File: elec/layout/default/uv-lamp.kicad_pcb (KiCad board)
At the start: 2 copper layers, 21 x 21 mm, 3 parts, among them U1 ?, U2 ?, U3 ?

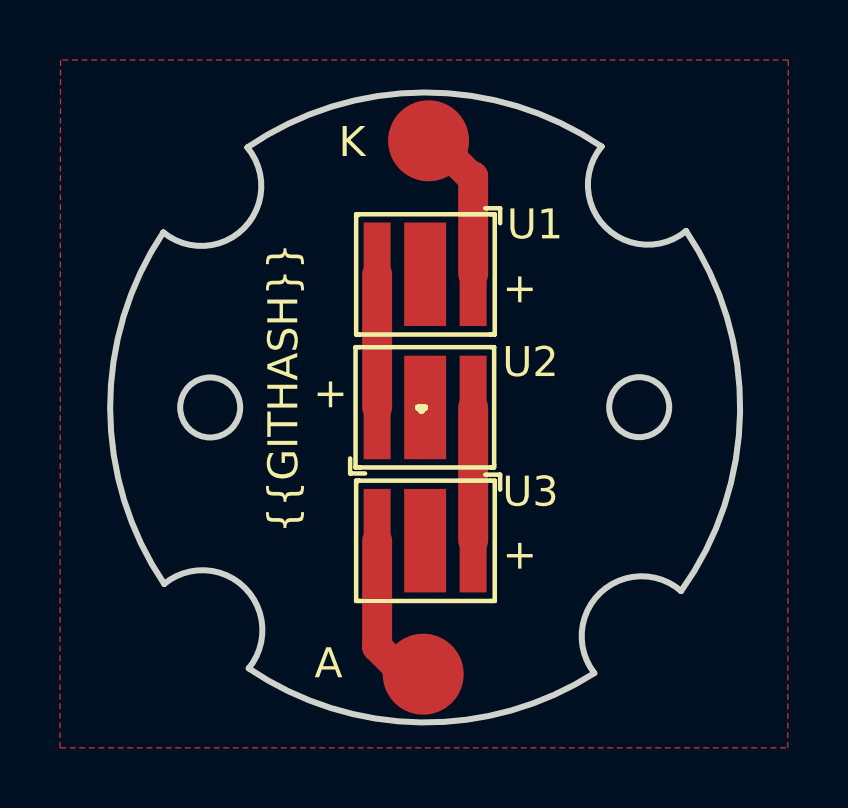
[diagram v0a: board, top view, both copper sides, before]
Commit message: ccdriver
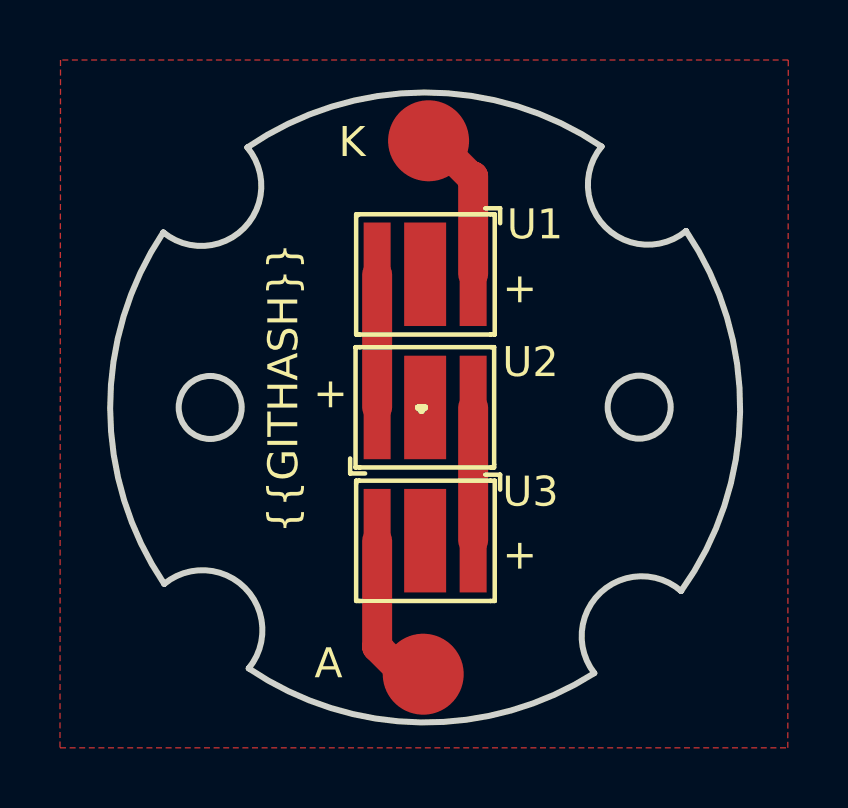
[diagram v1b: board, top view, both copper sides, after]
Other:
- outline, holes or cut-outs redrawn
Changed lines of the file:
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@@
 	(gr_circle
 		(center 140.175 83.310002)
-		(end 141.175 83.310002)
+		(end 141.225 83.310002)
 		(stroke
 			(width 0.2)
@@
 	(gr_circle
 		(center 154.475 83.3)
-		(end 155.475 83.3)
+		(end 155.525 83.3)
 		(stroke
 			(width 0.2)

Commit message: error checking
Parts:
- U1, U2, U3: value ? -> (none)
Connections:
- net led1-k renamed A-1
- net led2-k renamed K
- net vcc renamed A
- U1 pad 3: led1-_3 -> (no net)
- U2 pad 3: led2-_3 -> (no net)
- U3 pad 3: led3-_3 -> (no net)
